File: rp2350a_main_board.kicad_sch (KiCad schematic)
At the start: 84 parts, among them J1 USB_C_Receptacle_USB2.0_16P, J10 Conn_02x12, J2 SM03B-SRSS-TB, J3 Micro_SD_Card_Det1, J4 SM03B-SRSS-TB, J5 Conn_02x12, J6 Conn_02x12, J7 Conn_02x12, J8 Conn_02x12, J9 Conn_02x12, SW1 SW_SPDT, SW2 SW_Push, SW3 SW_Push, U1 TPS63802, U2 TPS2117DRL, U3 W25Q16JVSS, U4 RP2350_60QFN, U5 APS1604M-3SQRx-SN, U6 USBLC6-2SC6, Y1 ABM8-272-T3

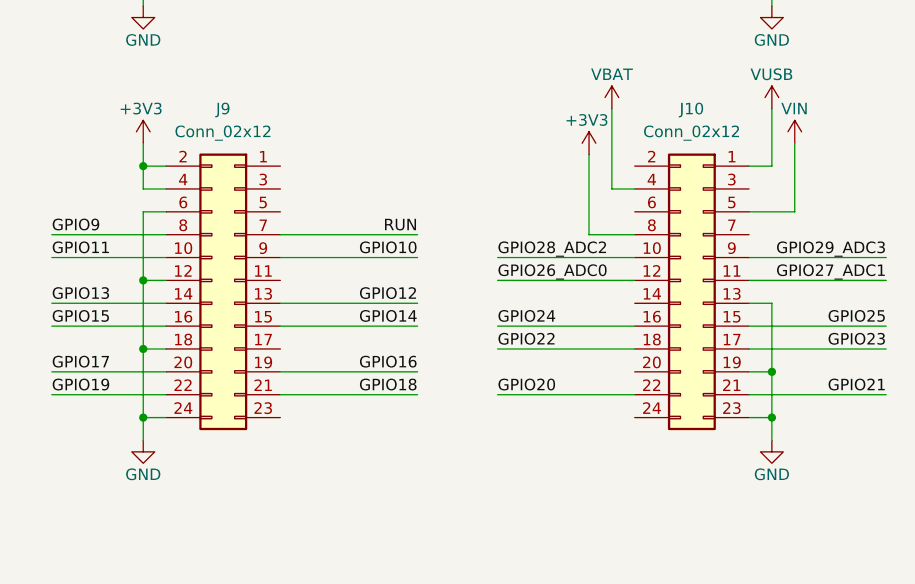
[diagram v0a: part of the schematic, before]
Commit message: v1.1.0 WIP
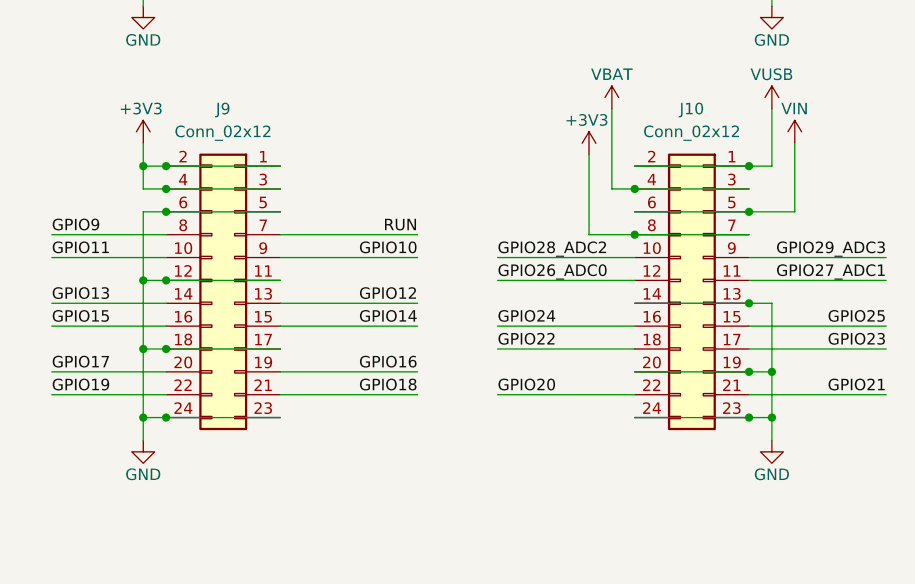
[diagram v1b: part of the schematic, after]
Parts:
- R15: footprint Resistor_SMD:R_0603_1608Metric_Pad0.98x0.95mm_HandSolder -> Resistor_SMD:R_0402_1005Metric_Pad0.72x0.64mm_HandSolder
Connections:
- net +3V3: now also J10.7 (Pin_7), J9.1 (Pin_1), J9.3 (Pin_3)
- net GND: now also J10.14 (Pin_14), J10.20 (Pin_20), J10.24 (Pin_24), J9.11 (Pin_11), J9.17 (Pin_17), J9.23 (Pin_23), J9.5 (Pin_5)
- net VBAT: now also J10.3 (Pin_3)
- net VIN: now also J10.6 (Pin_6)
- net VUSB: now also J10.2 (Pin_2)
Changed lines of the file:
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@@
 	)
 	(junction
+		(at 381 226.06)
+		(diameter 0)
+		(color 0 0 0 0)
+	)
+	(junction
 		(at 252.73 104.14)
 		(diameter 0)
@@
 	)
 	(junction
+		(at 381 203.2)
+		(diameter 0)
+		(color 0 0 0 0)
+	)
+	(junction
 		(at 199.39 104.14)
 		(diameter 0)
@@
 	)
 	(junction
+		(at 316.23 226.06)
+		(diameter 0)
+		(color 0 0 0 0)
+	)
+	(junction
 		(at 171.45 151.13)
 		(diameter 0)
@@
 	)
 	(junction
+		(at 316.23 200.66)
+		(diameter 0)
+		(color 0 0 0 0)
+	)
+	(junction
 		(at 381 129.54)
 		(diameter 0)
@@
 	)
 	(junction
+		(at 316.23 218.44)
+		(diameter 0)
+		(color 0 0 0 0)
+	)
+	(junction
 		(at 381 101.6)
 		(diameter 0)
@@
 	)
 	(junction
+		(at 368.3 200.66)
+		(diameter 0)
+		(color 0 0 0 0)
+	)
+	(junction
+		(at 381 198.12)
+		(diameter 0)
+		(color 0 0 0 0)
+	)
+	(junction
 		(at 101.6 111.76)
 		(diameter 0)
@@
 	)
 	(junction
+		(at 316.23 210.82)
+		(diameter 0)
+		(color 0 0 0 0)
+	)
+	(junction
 		(at 383.54 177.8)
 		(diameter 0)
@@
 	)
 	(junction
+		(at 381 220.98)
+		(diameter 0)
+		(color 0 0 0 0)
+	)
+	(junction
 		(at 49.53 224.79)
 		(diameter 0)
@@
 	)
 	(junction
+		(at 316.23 198.12)
+		(diameter 0)
+		(color 0 0 0 0)
+	)
+	(junction
 		(at 191.77 114.3)
 		(diameter 0)
@@
 	)
 	(junction
+		(at 316.23 203.2)
+		(diameter 0)
+		(color 0 0 0 0)
+	)
+	(junction
 		(at 49.53 161.29)
 		(diameter 0)
@@
 	)
 	(junction
+		(at 381 213.36)
+		(diameter 0)
+		(color 0 0 0 0)
+	)
+	(junction
 		(at 127 111.76)
 		(diameter 0)
@@
 		(color 0 0 0 0)
 	)
+	(junction
+		(at 368.3 205.74)
+		(diameter 0)
+		(color 0 0 0 0)
+	)
 	(no_connect
 		(at 72.39 58.42)
@@
 	(wire
 		(pts
+			(xy 368.3 205.74) (xy 381 205.74)
+		)
+		(stroke
+			(width 0)
+			(type default)
+		)
+	)
+	(wire
+		(pts
 			(xy 313.69 180.34) (xy 313.69 177.8)
 		)
@@
 	(wire
 		(pts
+			(xy 316.23 203.2) (xy 328.93 203.2)
+		)
+		(stroke
+			(width 0)
+			(type default)
+		)
+	)
+	(wire
+		(pts
 			(xy 313.69 149.86) (xy 316.23 149.86)
 		)
@@
 	(wire
 		(pts
+			(xy 368.3 213.36) (xy 381 213.36)
+		)
+		(stroke
+			(width 0)
+			(type default)
+		)
+	)
+	(wire
+		(pts
 			(xy 226.06 179.07) (xy 241.3 179.07)
 		)
@@
 	(wire
 		(pts
+			(xy 316.23 226.06) (xy 328.93 226.06)
+		)
+		(stroke
+			(width 0)
+			(type default)
+		)
+	)
+	(wire
+		(pts
 			(xy 313.69 101.6) (xy 316.23 101.6)
 		)
@@
 	(wire
 		(pts
+			(xy 368.3 200.66) (xy 381 200.66)
+		)
+		(stroke
+			(width 0)
+			(type default)
+		)
+	)
+	(wire
+		(pts
+			(xy 316.23 198.12) (xy 328.93 198.12)
+		)
+		(stroke
+			(width 0)
+			(type default)
+		)
+	)
+	(wire
+		(pts
 			(xy 316.23 205.74) (xy 303.53 205.74)
 		)
@@
 	(wire
 		(pts
+			(xy 368.3 203.2) (xy 381 203.2)
+		)
+		(stroke
+			(width 0)
+			(type default)
+		)
+	)
+	(wire
+		(pts
 			(xy 50.8 55.88) (xy 72.39 55.88)
 		)
@@
 	(wire
 		(pts
+			(xy 368.3 220.98) (xy 381 220.98)
+		)
+		(stroke
+			(width 0)
+			(type default)
+		)
+	)
+	(wire
+		(pts
 			(xy 316.23 223.52) (xy 303.53 223.52)
 		)
@@
 	(wire
 		(pts
+			(xy 316.23 210.82) (xy 328.93 210.82)
+		)
+		(stroke
+			(width 0)
+			(type default)
+		)
+	)
+	(wire
+		(pts
 			(xy 226.06 247.65) (xy 241.3 247.65)
 		)
@@
 	(wire
 		(pts
+			(xy 316.23 218.44) (xy 328.93 218.44)
+		)
+		(stroke
+			(width 0)
+			(type default)
+		)
+	)
+	(wire
+		(pts
 			(xy 50.8 269.24) (xy 50.8 264.16)
 		)
@@
 	(wire
 		(pts
+			(xy 316.23 200.66) (xy 328.93 200.66)
+		)
+		(stroke
+			(width 0)
+			(type default)
+		)
+	)
+	(wire
+		(pts
 			(xy 199.39 99.06) (xy 199.39 104.14)
 		)
@@
 	(wire
 		(pts
+			(xy 368.3 198.12) (xy 381 198.12)
+		)
+		(stroke
+			(width 0)
+			(type default)
+		)
+	)
+	(wire
+		(pts
 			(xy 256.54 58.42) (xy 279.4 58.42)
 		)
@@
 	(wire
 		(pts
+			(xy 368.3 226.06) (xy 381 226.06)
+		)
+		(stroke
+			(width 0)
+			(type default)
+		)
+	)
+	(wire
+		(pts
 			(xy 35.56 68.58) (xy 35.56 66.04)
 		)
@@
 			)
 		)
-		(property "Footprint" "Resistor_SMD:R_0603_1608Metric_Pad0.98x0.95mm_HandSolder"
+		(property "Footprint" "Resistor_SMD:R_0402_1005Metric_Pad0.72x0.64mm_HandSolder"
 			(at 213.36 64.008 90)
 			(effects

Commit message: Update BOM
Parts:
- J1: now in the parts list
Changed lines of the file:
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@@
 		(unit 1)
 		(exclude_from_sim no)
-		(in_bom no)
+		(in_bom yes)
 		(on_board yes)
 		(dnp no)
